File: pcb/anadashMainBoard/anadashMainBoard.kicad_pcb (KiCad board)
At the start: 2 copper layers, 100 x 50 mm, 21 parts, among them J1 DisplayConnector, J2 LeftKeyConnector, J3 RightKeyConnector, J4 EncoderConnector

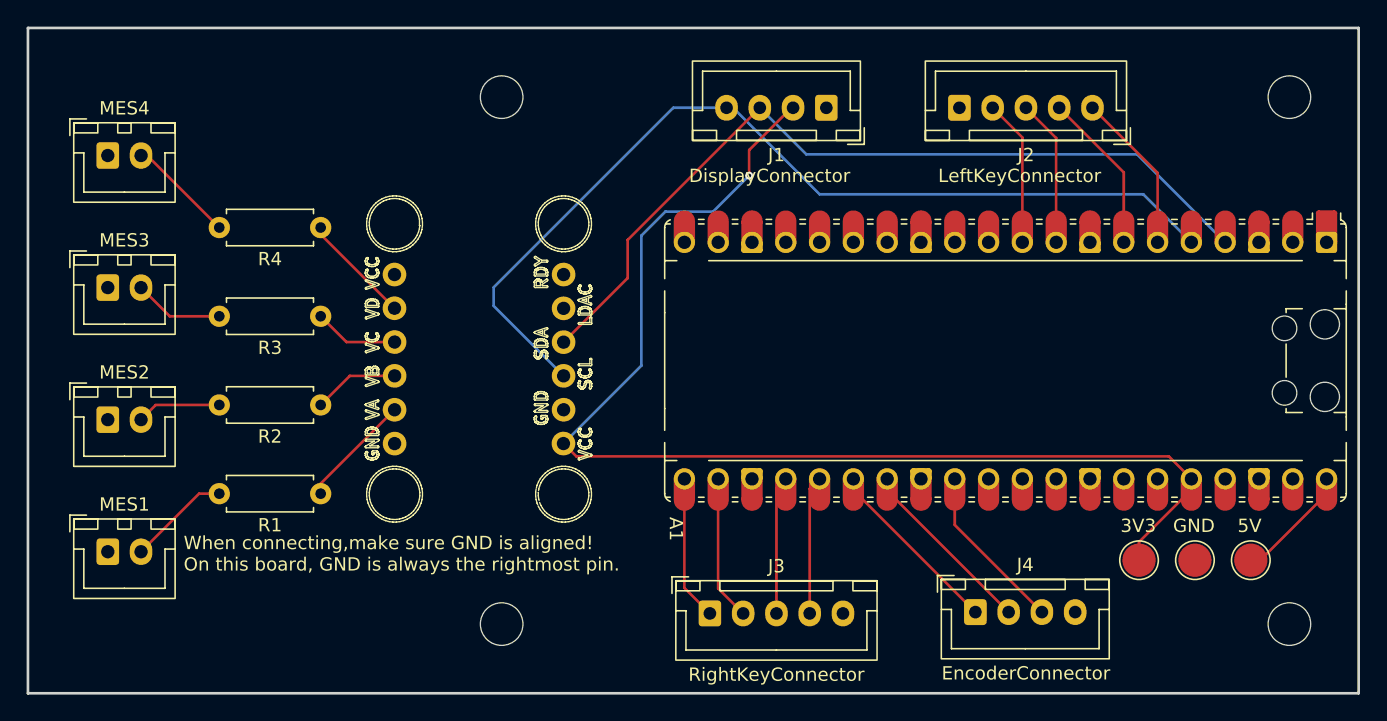
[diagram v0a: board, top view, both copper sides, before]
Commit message: added 3d files, or so I hopew
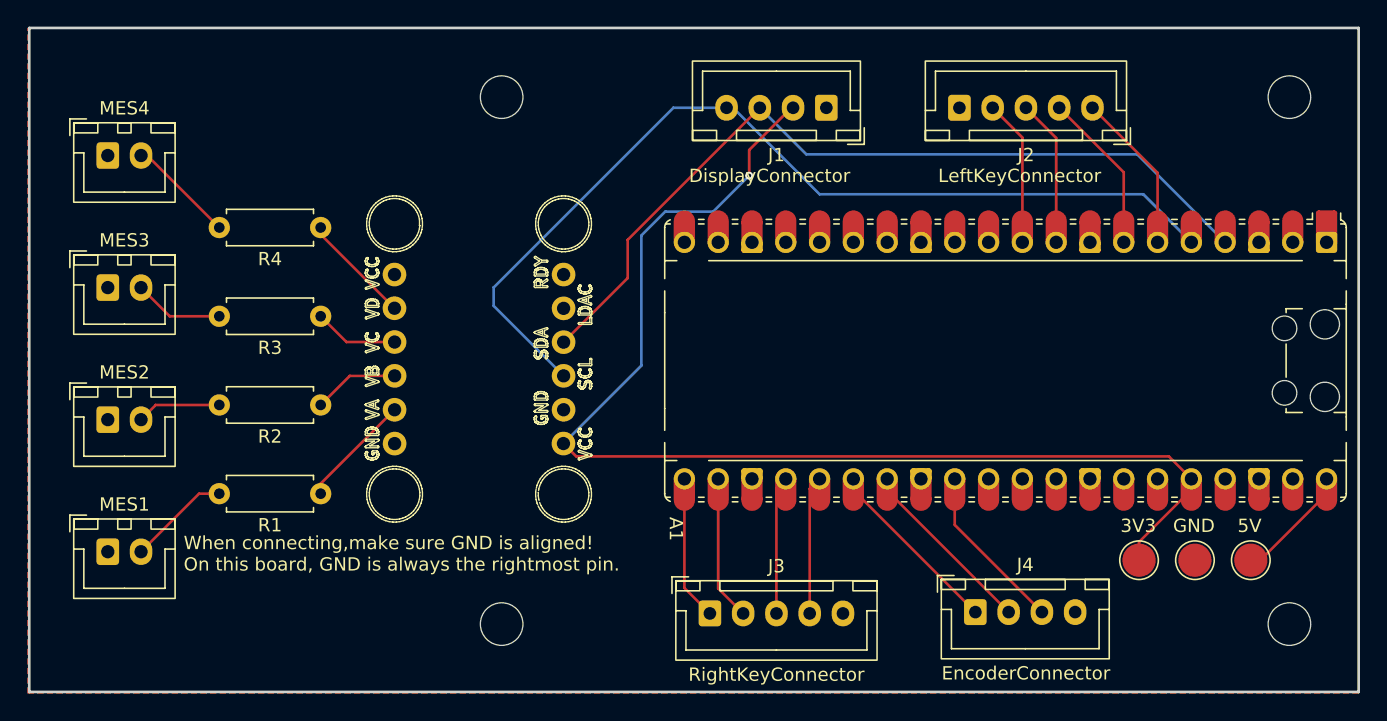
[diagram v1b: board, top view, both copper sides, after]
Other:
- board size 100 x 50 mm -> 99.9 x 49.9 mm
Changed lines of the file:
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@@
 		(capping no)
 		(filling no)
+		(grid_origin 108 120)
 		(pcbplotparams
 			(layerselection 0x00000000_00000000_55555555_5755f5ff)
@@
 	)
 	(gr_rect
-		(start 108 70)
-		(end 208 120)
+		(start 108.1 70)
+		(end 208 119.9)
 		(stroke
 			(width 0.2)
@@
 	)
 	(segment
-		(start 153.07 88.798825)
-		(end 153.07 85.93)
+		(start 131.938459 93.605126)
+		(end 130 91.666667)
 		(width 0.2)
 		(layer "F.Cu")
-		(net "SDA")
+		(net "Net-(U1-VC)")
 	)
 	(segment
-		(start 153.07 85.93)
-		(end 163 76)
+		(start 135.555699 93.605126)
+		(end 131.938459 93.605126)
 		(width 0.2)
 		(layer "F.Cu")
-		(net "SDA")
+		(net "Net-(U1-VC)")
 	)
 	(segment
-		(start 148.255699 93.613126)
-		(end 153.07 88.798825)
+		(start 135.546699 91.065126)
+		(end 130 85.518427)
 		(width 0.2)
 		(layer "F.Cu")
-		(net "SDA")
-	)
-	(segment
-		(start 166.5 79.5)
-		(end 191.3625 79.5)
-		(width 0.2)
-		(layer "B.Cu")
-		(net "SDA")
-	)
-	(segment
-		(start 163 76)
-		(end 166.5 79.5)
-		(width 0.2)
-		(layer "B.Cu")
-		(net "SDA")
+		(net "Net-(U1-VD)")
 	)
 	(segment
-		(start 191.3625 79.5)
-		(end 197.9725 86.11)
+		(start 130 85.518427)
+		(end 130 85)
 		(width 0.2)
-		(layer "B.Cu")
-		(net "SDA")
+		(layer "F.Cu")
+		(net "Net-(U1-VD)")
 	)
 	(segment
@@
 	)
 	(segment
+		(start 153.07 88.798825)
+		(end 153.07 85.93)
+		(width 0.2)
+		(layer "F.Cu")
+		(net "SDA")
+	)
+	(segment
+		(start 153.07 85.93)
+		(end 163 76)
+		(width 0.2)
+		(layer "F.Cu")
+		(net "SDA")
+	)
+	(segment
+		(start 148.255699 93.613126)
+		(end 153.07 88.798825)
+		(width 0.2)
+		(layer "F.Cu")
+		(net "SDA")
+	)
+	(segment
+		(start 166.5 79.5)
+		(end 191.3625 79.5)
+		(width 0.2)
+		(layer "B.Cu")
+		(net "SDA")
+	)
+	(segment
+		(start 163 76)
+		(end 166.5 79.5)
+		(width 0.2)
+		(layer "B.Cu")
+		(net "SDA")
+	)
+	(segment
+		(start 191.3625 79.5)
+		(end 197.9725 86.11)
+		(width 0.2)
+		(layer "B.Cu")
+		(net "SDA")
+	)
+	(segment
 		(start 192.8925 80.8925)
 		(end 192.8925 86.11)
@@
 	)
 	(segment
-		(start 131.938459 93.605126)
-		(end 130 91.666667)
-		(width 0.2)
-		(layer "F.Cu")
-		(net "Net-(U1-VC)")
-	)
-	(segment
-		(start 135.555699 93.605126)
-		(end 131.938459 93.605126)
-		(width 0.2)
-		(layer "F.Cu")
-		(net "Net-(U1-VC)")
-	)
-	(segment
-		(start 135.546699 91.065126)
-		(end 130 85.518427)
-		(width 0.2)
-		(layer "F.Cu")
-		(net "Net-(U1-VD)")
-	)
-	(segment
-		(start 130 85.518427)
-		(end 130 85)
-		(width 0.2)
-		(layer "F.Cu")
-		(net "Net-(U1-VD)")
-	)
-	(segment
